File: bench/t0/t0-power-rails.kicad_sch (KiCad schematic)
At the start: 29 parts, among them J1 POINTER — USB-C 5 V in (charg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, J2 WEARABLE — USB-C 5 V in (char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, M1 Multimeter inline (mA), M2 Multimeter inline (mA), SW1 Slide switch (load on/off), SW2 Slide switch (load on/off), U1 TP4056-C charge/protect 1 A, U10 MAX98357A (I²S amp, L), U11 MAX98357A (I²S amp, R), U12 OV2640 160° (cam L), U13 OV2640 160° (cam R), U2 ESP32-S3-DevKitC-1 N16R8 (poi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, U3 BNO085 breakout (IMU), U4 VL53L1X + optical cover (ToF), U5 DWM3000 (UWB tag), U6 TP4056-C charge/protect 1 A, U7 ESP32-S3-DevKitC-1 N16R8 (wea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, U8 BNO085 breakout (head IMU), U9 DWM3000 (UWB anchor)

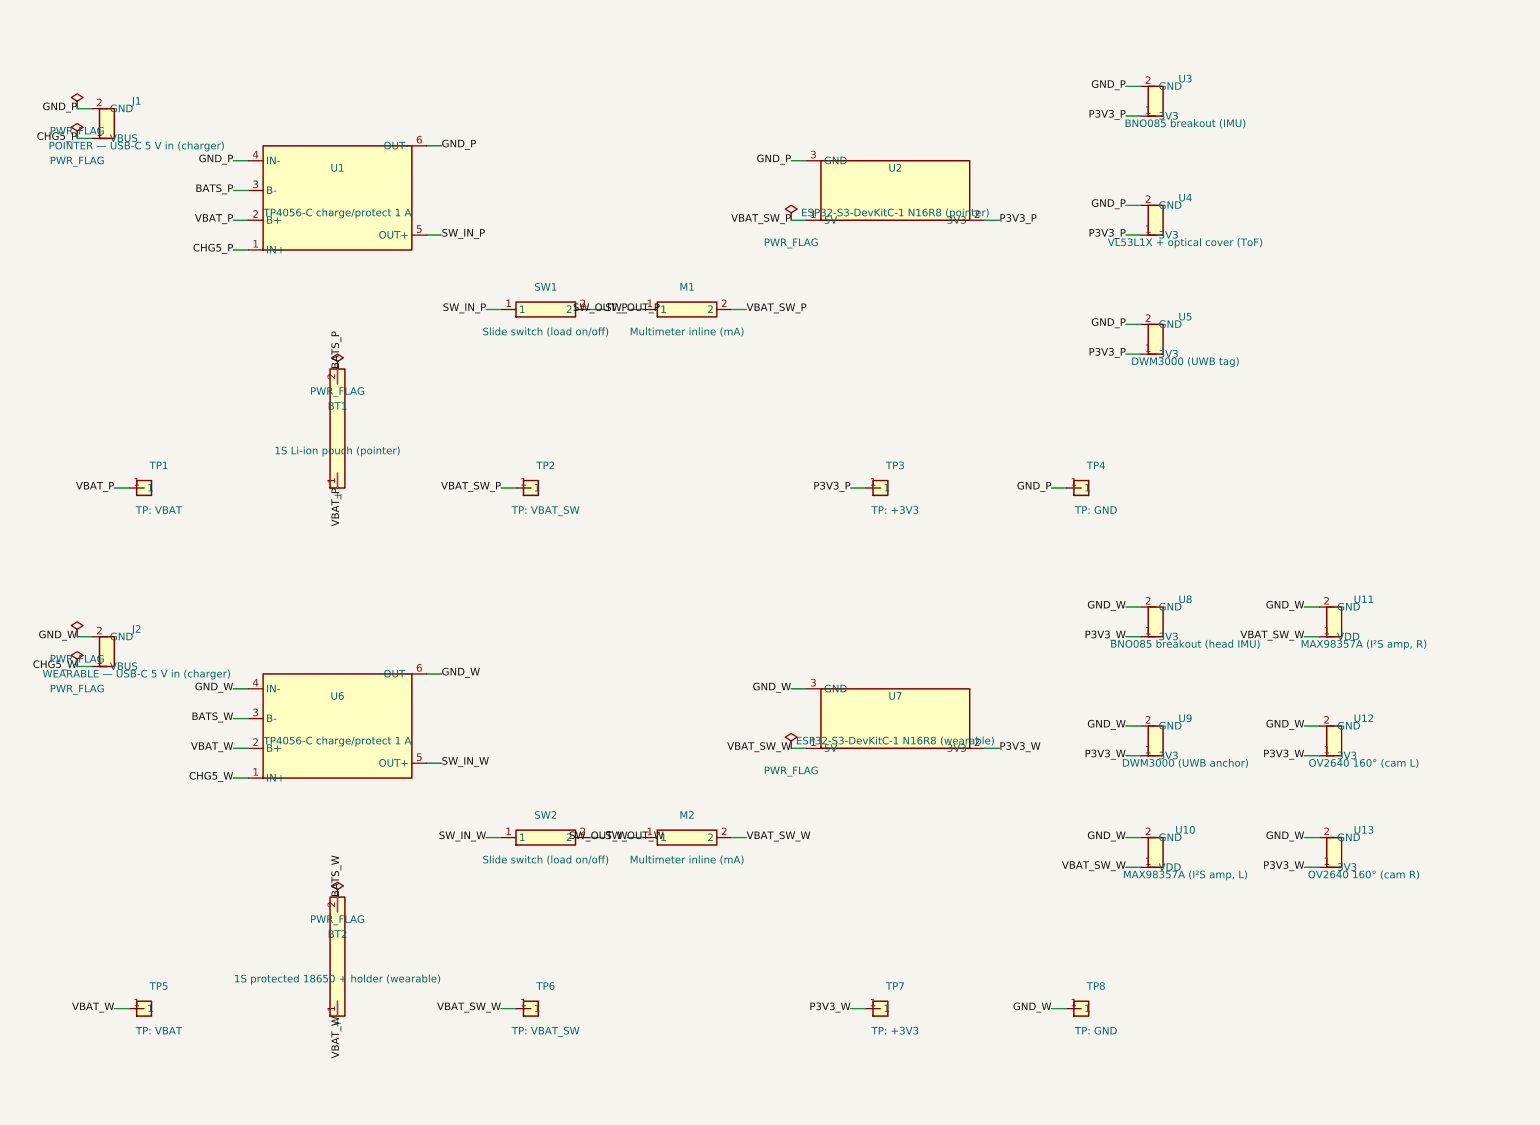
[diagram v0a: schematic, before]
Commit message: bench t0
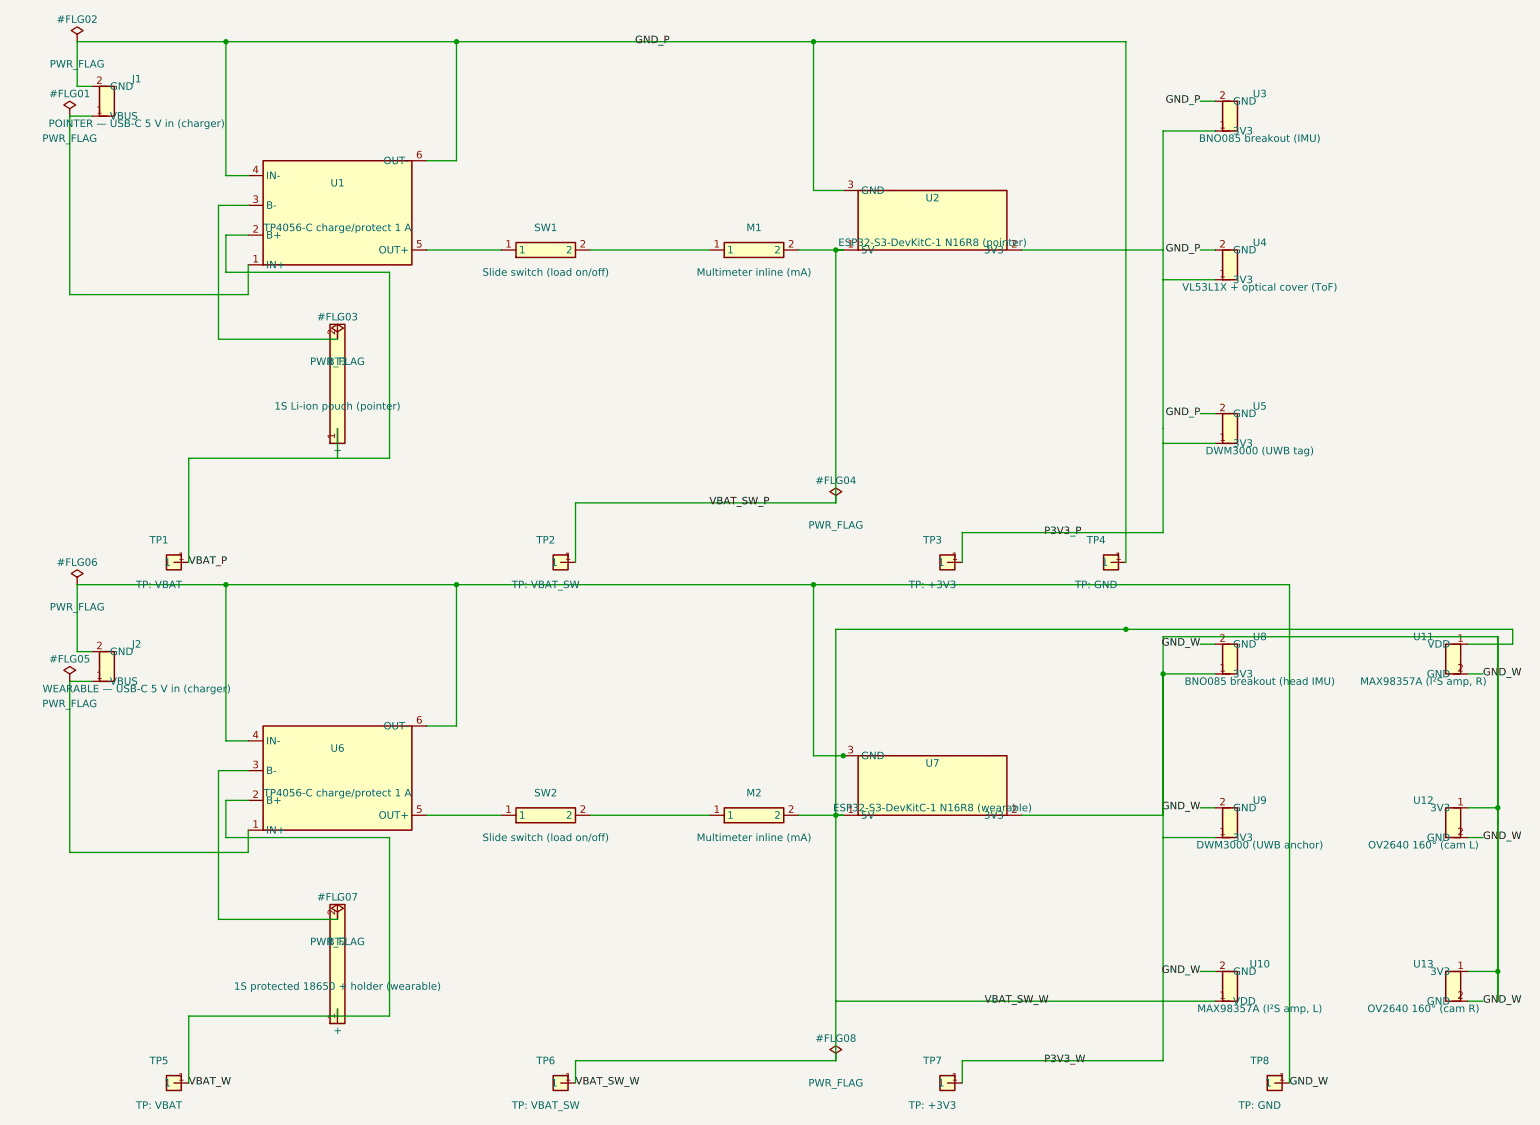
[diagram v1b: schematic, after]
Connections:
- net BATS_P: no longer names the net of BT1.2 (-), U1.3 (B-)
- net BATS_W: no longer names the net of BT2.2 (-), U6.3 (B-)
- net CHG5_P: no longer names the net of J1.1 (VBUS), U1.1 (IN+)
- net CHG5_W: no longer names the net of J2.1 (VBUS), U6.1 (IN+)
- net SW_IN_P: no longer names the net of SW1.1, U1.5 (OUT+)
- net SW_IN_W: no longer names the net of SW2.1, U6.5 (OUT+)
- net SW_OUT_P: no longer names the net of M1.1, SW1.2
- net SW_OUT_W: no longer names the net of M2.1, SW2.2
